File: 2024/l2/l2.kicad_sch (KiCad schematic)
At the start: 20 parts, among them J1 Conn_01x04, J2 Conn_01x02, J3 Conn_01x04, U5 DEV-15583

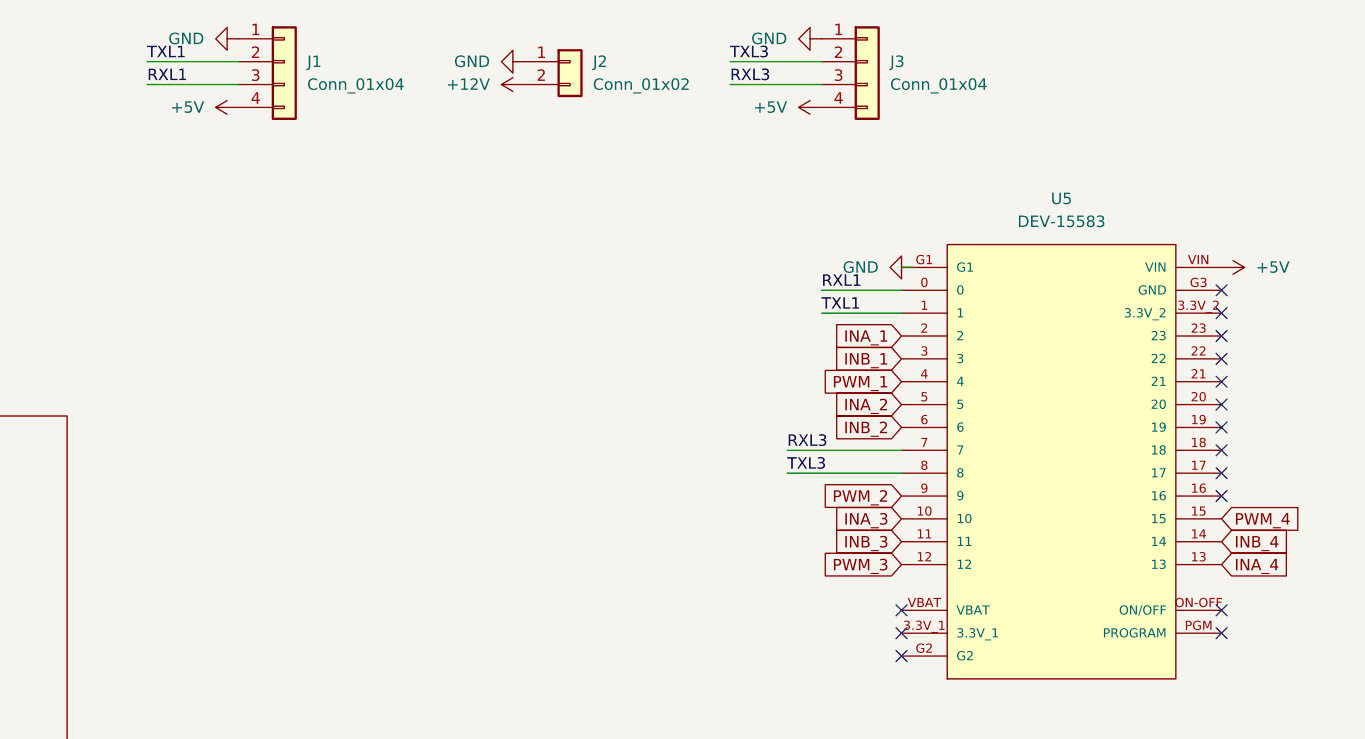
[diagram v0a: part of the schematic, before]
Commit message: final 0.9
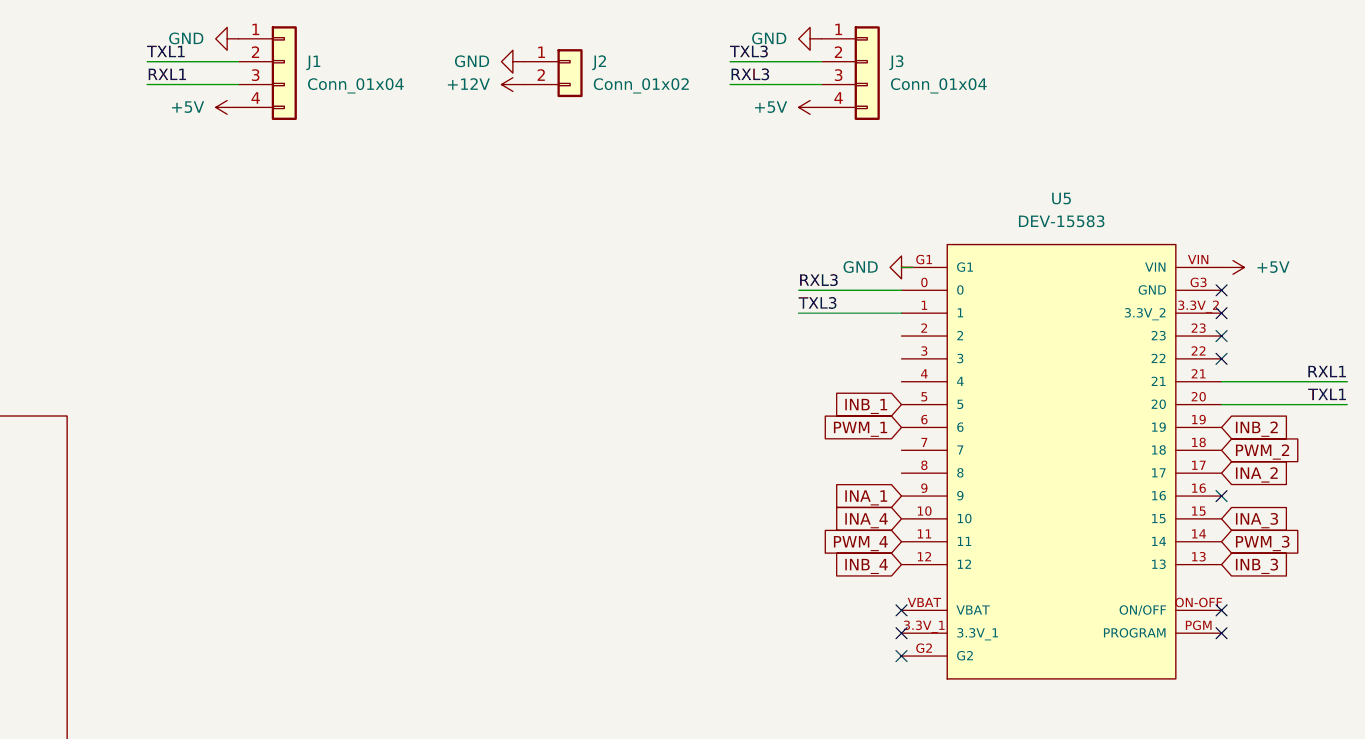
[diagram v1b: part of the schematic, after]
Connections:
- net INA_1: now also U5.9; no longer U5.2
- net INA_2: now also U5.17; no longer U5.5
- net INA_3: now also U5.15; no longer U5.10
- net INA_4: now also U5.10; no longer U5.13
- net INB_1: now also U5.5; no longer U5.3
- net INB_2: now also U5.19; no longer U5.6
- net INB_3: now also U5.13; no longer U5.11
- net INB_4: now also U5.12; no longer U5.14
- net PWM_1: now also U5.6; no longer U5.4
- net PWM_2: now also U5.18; no longer U5.9
- net PWM_3: now also U5.14; no longer U5.12
- net PWM_4: now also U5.11; no longer U5.15
- net RXL1: now also U5.21; no longer U5.0
- net RXL3: now also U5.0; no longer U5.7
- net TXL1: now also U5.20; no longer U5.1
- net TXL3: now also U5.1; no longer U5.8
- no-connect marks 31 -> 26
